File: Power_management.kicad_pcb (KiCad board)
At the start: 2 copper layers, 186 x 135 mm, 15 parts, among them J15 USB_C_Receptacle, Q1 BSS84, Q2 BSS84, Q7 AO3401A, Q8 BUK7M67-60EX, Q9 BUK7M67-60EX, U1 BQ78350DBT, U3 BQ76920PW, U4 TVS2200DRV, U5 BQ76200PW

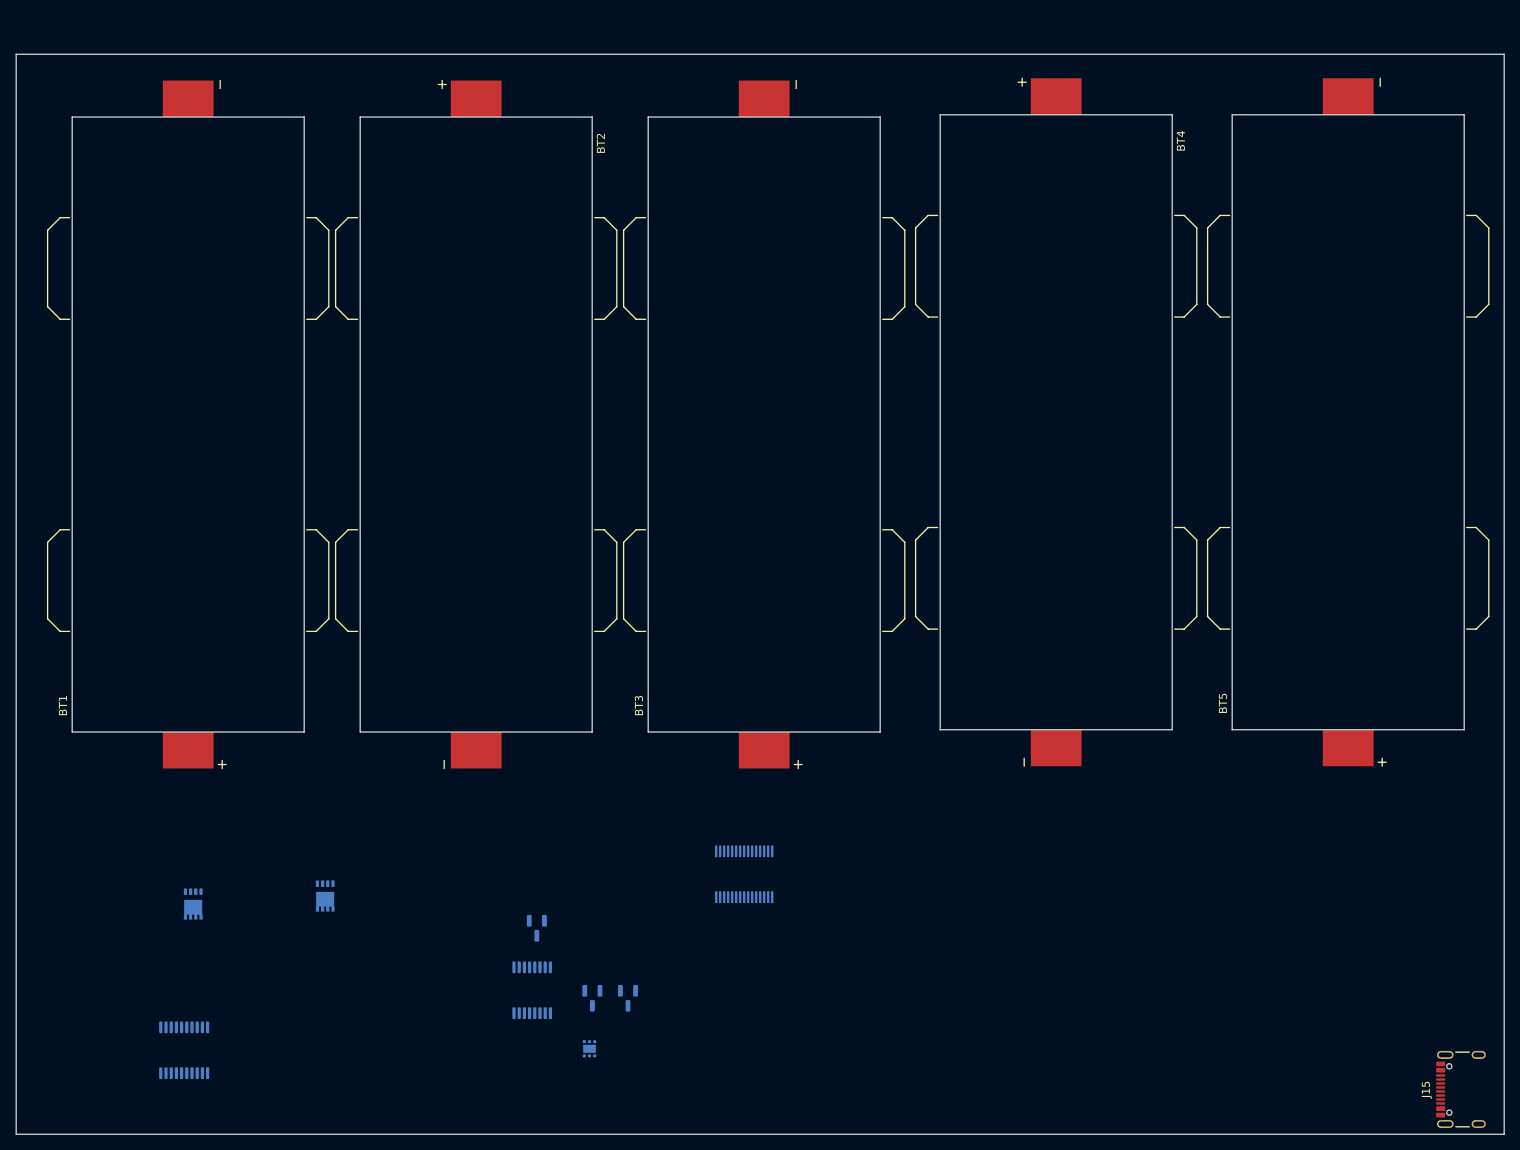
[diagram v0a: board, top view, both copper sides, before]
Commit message: progress
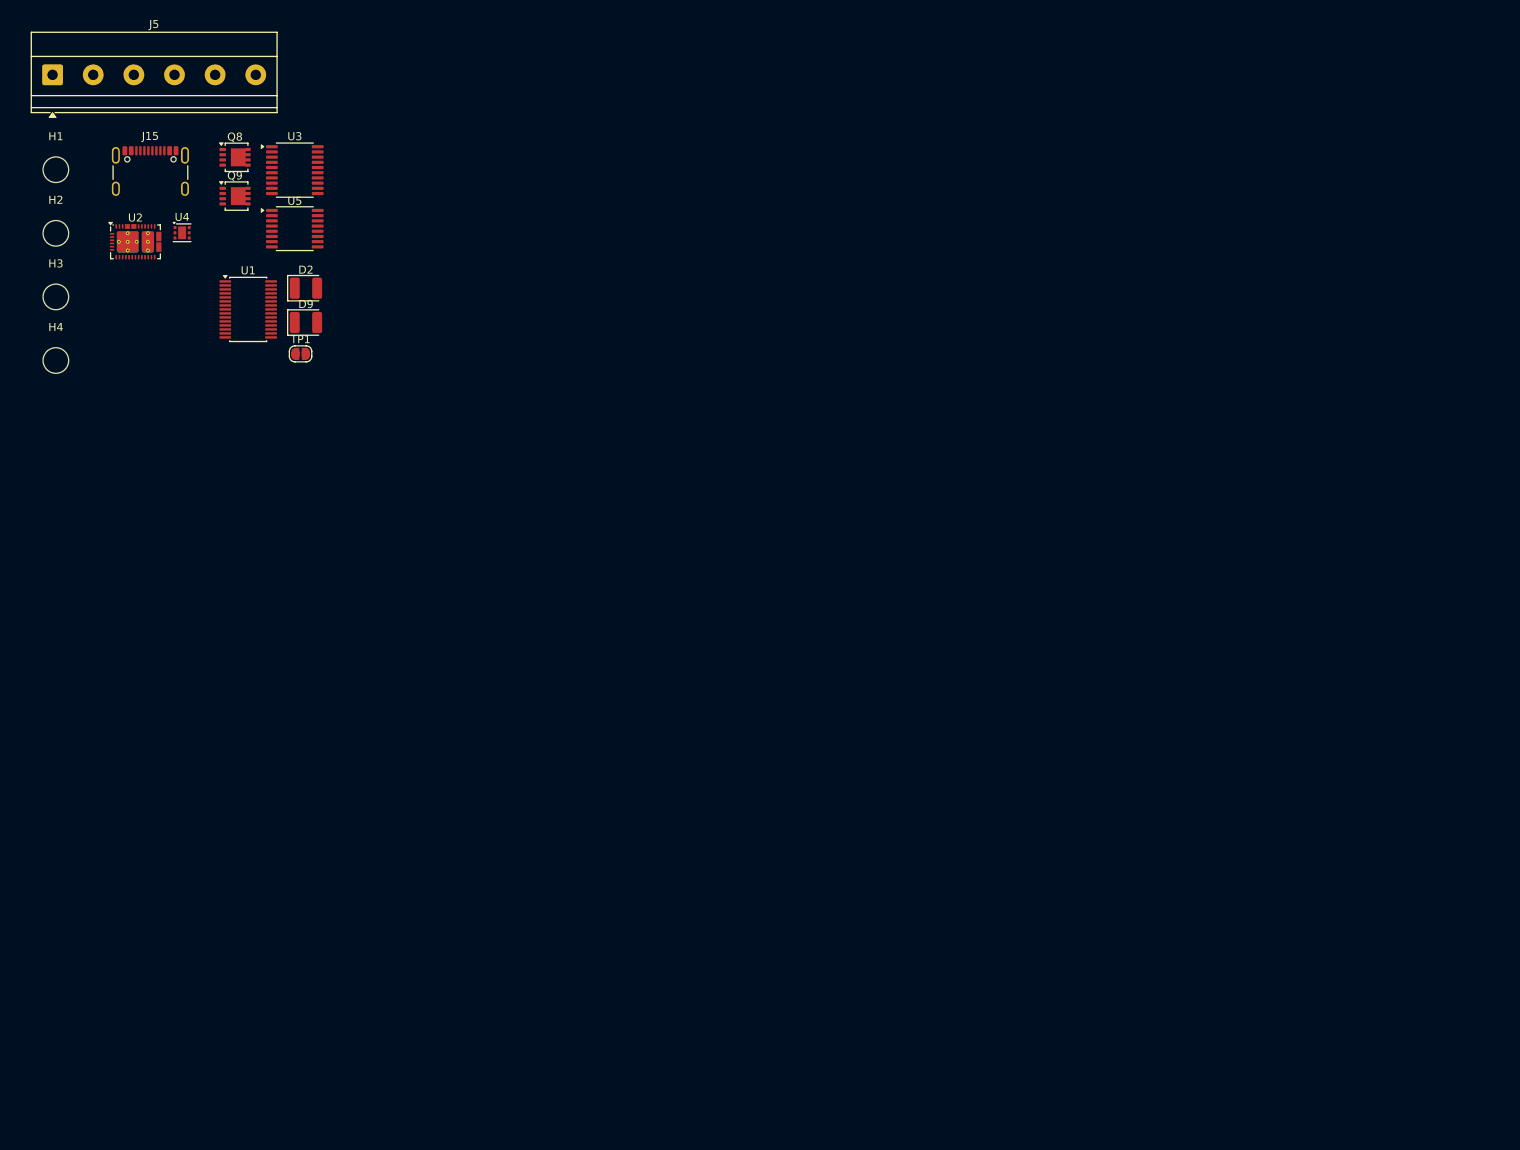
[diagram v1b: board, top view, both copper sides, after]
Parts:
- removed BT1, BT2, BT3, BT4, BT5: 1106, 26650_cell_holder:BAT_1106
- removed Q1, Q2: BSS84, Package_TO_SOT_SMD:SOT-23
- removed Q7: AO3401A, Package_TO_SOT_SMD:SOT-23
- added D2: 599-2100-137F, LED_SMD:LED_1210_3225Metric, F.Cu at (60.2, 52.2)
- added D9: 599-2100-137F, LED_SMD:LED_1210_3225Metric, F.Cu at (60.2, 56.5)
- added H1: MountingHole, MountingHole:MountingHole_3.2mm_M3, F.Cu at (29.0, 37.4)
- added H2: MountingHole, MountingHole:MountingHole_3.2mm_M3, F.Cu at (29.0, 45.4)
- added H3: MountingHole, MountingHole:MountingHole_3.2mm_M3, F.Cu at (29.0, 53.3)
- added H4: MountingHole, MountingHole:MountingHole_3.2mm_M3, F.Cu at (29.0, 61.3)
- added J5: Conn_01x06, TerminalBlock_Phoenix:TerminalBlock_Phoenix_MKDS-1,5-6-5.08_1x06_P5.08mm_Horizontal, F.Cu at (28.5, 25.6)
- added TP1: TestPoint_2Pole, Jumper:SolderJumper-2_P1.3mm_Open_RoundedPad1.0x1.5mm, F.Cu at (59.5, 60.5)
- added U2: TPS25730D, Package_DFN_QFN:Texas_REF0038A_WQFN-38-2EP_6x4mm_P0.4, F.Cu at (38.9, 46.4)
- Q8, Q9, U1, U3, U4, U5: moved to F.Cu
- moved J15 200.3 mm to (40.8, 38.7), turned to 0 degrees
- moved U4 114.0 mm to (44.7, 45.3), turned to 0 degrees
- moved U3 110.9 mm to (58.8, 37.5), turned to 0 degrees
- moved U5 99.7 mm to (58.8, 44.8), turned to 0 degrees
- moved U1 94.0 mm to (53.0, 54.9), turned to 0 degrees
- moved Q8 93.5 mm to (51.3, 35.9), turned to 0 degrees
- moved Q9 88.2 mm to (51.3, 40.7), turned to 0 degrees
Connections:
- J15 pad A5: unconnected-(J15-CC1-PadA5) -> /USB Interface/CC1
- J15 pad B5: unconnected-(J15-CC2-PadB5) -> /USB Interface/CC2
- Q8 pad 1: Net-(Q8-S-Pad1) -> /Cell Monitor/Top_cell_stack
- Q8 pad 2: Net-(Q8-S-Pad1) -> /Cell Monitor/Top_cell_stack
- Q8 pad 3: Net-(Q8-S-Pad1) -> /Cell Monitor/Top_cell_stack
- U1 pad 11: unconnected-(U1-SMBD-Pad11) -> /Cell Controller/SMBD
- U1 pad 12: unconnected-(U1-VEN-Pad12) -> /Cell Controller/VEN
- U1 pad 13: unconnected-(U1-SMBC-Pad13) -> /Cell Controller/SMBC
- U1 pad 14: Net-(U1-~{DISP}) -> GND
- U1 pad 15: unconnected-(U1-PWRM-Pad15) -> /Cell Controller/PWRM
- U1 pad 16: unconnected-(U1-LED1-Pad16) -> /Cell Controller/LED1
- U1 pad 17: unconnected-(U1-LED2-Pad17) -> /Cell Controller/LED2
- U1 pad 18: unconnected-(U1-LED3-Pad18) -> /Cell Controller/LED3
- U1 pad 19: unconnected-(U1-LED4-Pad19) -> /Cell Controller/LED4
- U1 pad 20: unconnected-(U1-LED5-Pad20) -> /Cell Controller/LED5
- U1 pad 21: unconnected-(U1-GPIO_A-Pad21) -> /Cell Controller/HS_SW_CP_EN
- U1 pad 27: unconnected-(U1-RBI-Pad27) -> Net-(U1-RBI)
- U1 pad 28: unconnected-(U1-GPIO_B-Pad28) -> /Cell Controller/HS_SW_PMON_EN
- U1 pad 30: unconnected-(U1-SMBA-Pad30) -> GND
- U1 pad 5: unconnected-(U1-~{PRECHG}-Pad5) -> /Cell Controller/HS_SW_PCHG_EN
- U1 pad 7: unconnected-(U1-BAT-Pad7) -> /Cell Controller/BAT
- U3 pad 17: Net-(U3-VC0) -> GND
- U3 pad 9: /Cell Monitor/REGSRC -> /Cell Monitor/BAT
- U5 pad 14: /Cell Monitor/PCHG_GATE -> unconnected-(U5-PCHG-Pad14)
- U5 pad 5: /Cell Monitor/HS_SW_CP_EN -> /Cell Controller/HS_SW_CP_EN
- U5 pad 7: /Cell Monitor/HS_SW_PMON_EN -> /Cell Controller/HS_SW_PMON_EN
- U5 pad 8: /Cell Monitor/HS_SW_PCHG_EN -> /Cell Controller/HS_SW_PCHG_EN
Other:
- board outline removed
